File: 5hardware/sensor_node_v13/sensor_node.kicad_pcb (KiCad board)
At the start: 2 copper layers, 24 x 48 mm, 43 parts, among them J1 Conn_01x08_Socket, J2 Conn_01x08_Socket, Q1 AO3400A, Q2 AO3401A, Q4 AO3401A, SW1 SW_Push, SW2 SW_Push, SW3 SW_Push, SW4 SW_Reed, SW5 SW_Push, SW6 SW_Push, SW7 SW_Push, U1 ESP-12F, U12 APDS-9960, U13 SHT31-DIS, U17 BH1750FVI-TR, U2 2N7002DW, U3 INA219AxDCN, U7 XC6206PxxxMR, U8 TPL5110

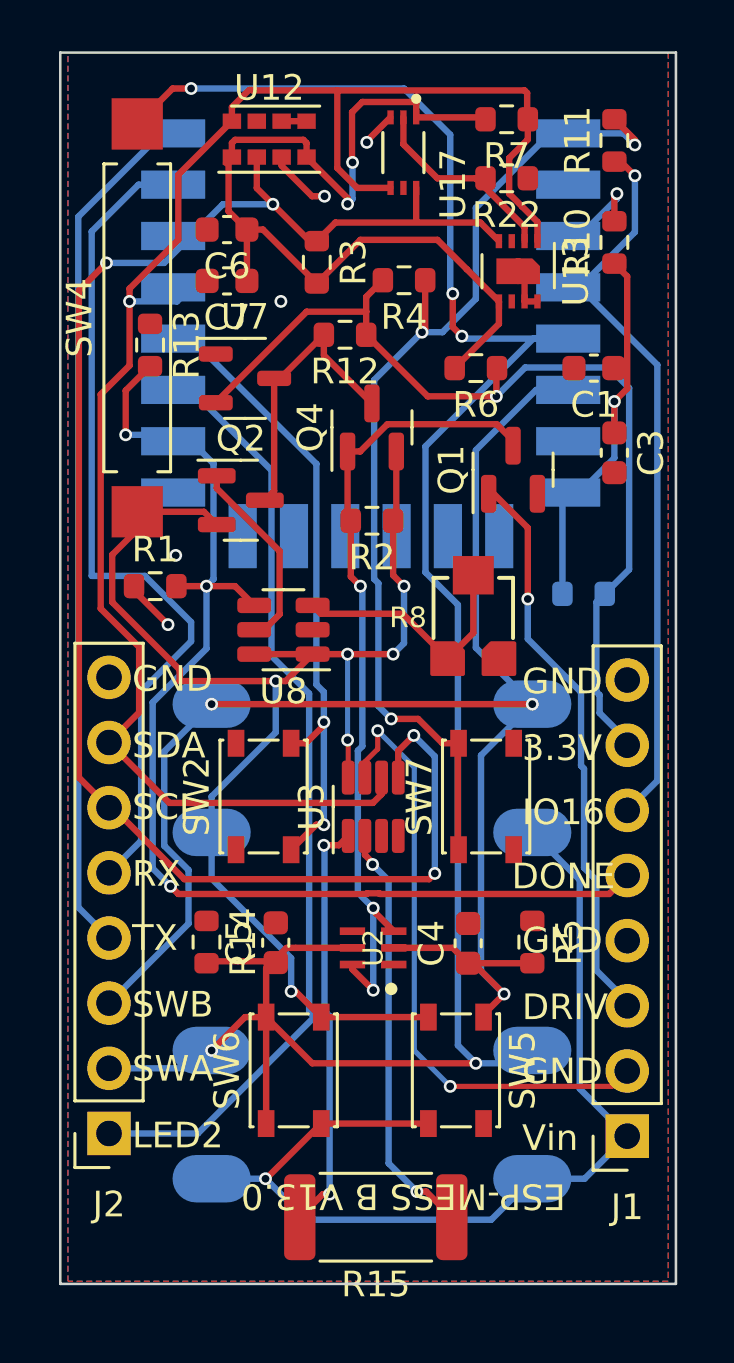
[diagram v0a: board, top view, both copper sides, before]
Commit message: updated PCB.
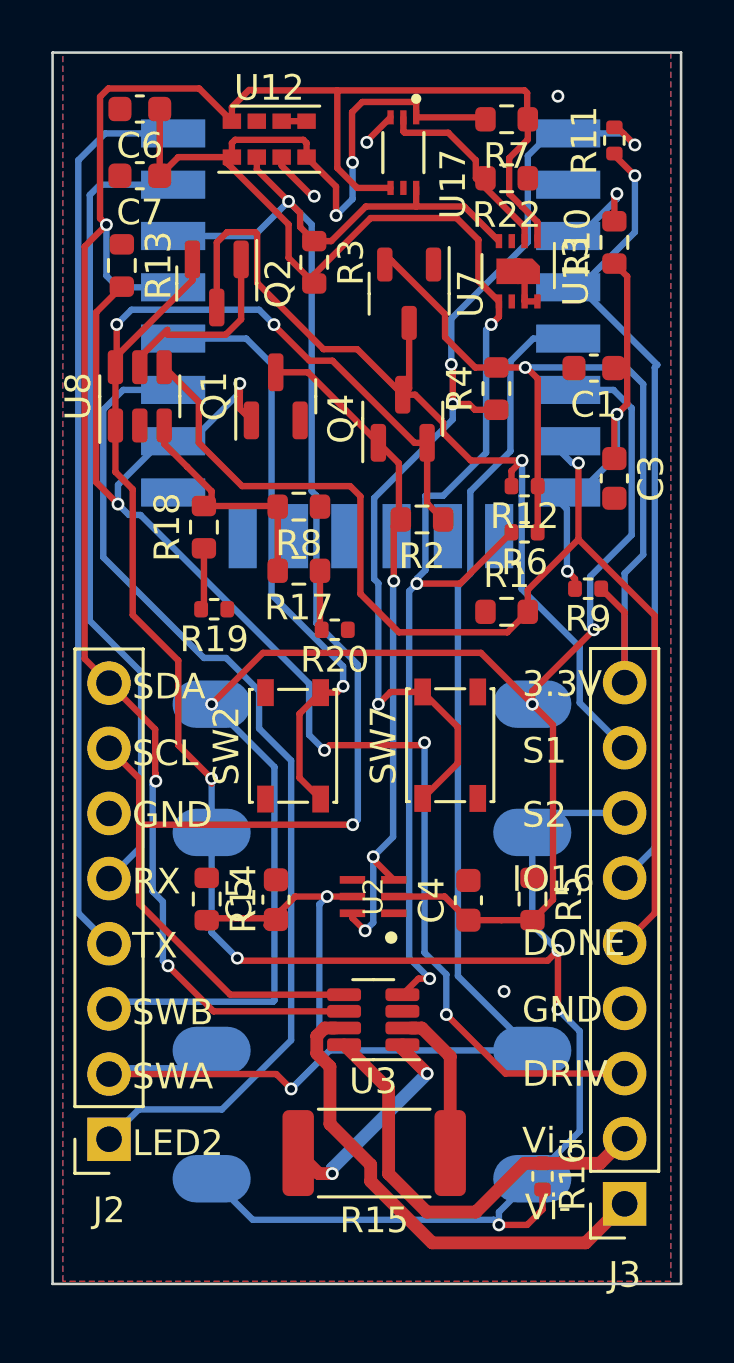
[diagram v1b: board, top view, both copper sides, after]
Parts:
- removed J1: Conn_01x08_Socket, Connector_PinSocket_2.54mm:PinSocket_1x08_P2.54mm_Vertical
- removed SW4: SW_Reed, Button_Switch_SMD:SW_SPST_REED_CT10-XXXX-G1
- removed SW5, SW6: SW_Push, Button_Switch_SMD:SW_SPST_PTS810
- added J3: Conn_01x09_Socket, Connector_PinSocket_2.54mm:PinSocket_1x09_P2.54mm_Vertical, F.Cu at (134.7, 98.8)
- added R16: 0K, Resistor_SMD:R_0402_1005Metric, F.Cu at (131.5, 97.7)
- added R17: R, Resistor_SMD:R_0603_1608Metric, F.Cu at (122.0, 74.1)
- added R18: R, Resistor_SMD:R_0603_1608Metric, F.Cu at (118.3, 72.4)
- added R19: 0K, Resistor_SMD:R_0402_1005Metric, F.Cu at (118.7, 75.6)
- added R20: 0K, Resistor_SMD:R_0402_1005Metric, F.Cu at (123.4, 76.4)
- R11, R12, R6: footprint Resistor_SMD:R_0603_1608Metric -> Resistor_SMD:R_0402_1005Metric
- R8: value EVM3ESX50B12 -> R; footprint EVM3ES:EMV3ESX50B12 -> Resistor_SMD:R_0603_1608Metric
- R9: footprint Resistor_SMD:R_0603_1608Metric -> Resistor_SMD:R_0402_1005Metric; moved to F.Cu
- moved R1 13.7 mm to (130.1, 75.7)
- moved U8 10.7 mm to (115.8, 67.3), turned to 90 degrees
- moved Q1 9.68 mm to (121.1, 67.3)
- moved R12 9.15 mm to (130.8, 70.8)
- moved Q2 8.50 mm to (118.8, 62.9), turned to -90 degrees
- moved U3 8.30 mm to (124.9, 91.6), turned to 180 degrees
- moved R8 8.06 mm to (122.0, 71.6), turned to 180 degrees
- moved U7 7.20 mm to (126.3, 63.3), turned to -90 degrees
- moved R6 6.68 mm to (130.8, 72.6)
- moved C6 5.80 mm to (115.8, 56.1)
- moved R4 5.55 mm to (129.7, 67.0), turned to 90 degrees
- moved C7 5.33 mm to (115.8, 58.7)
- moved R13 3.29 mm to (115.1, 62.2)
- moved R15 2.50 mm to (124.9, 96.8)
- moved SW7 2.44 mm to (127.9, 80.9)
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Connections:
- net Net-(Q2-D) renamed S1
- J2 pad 6: SCL -> GND
- J2 pad 7: SDA -> SCL
- J2 pad 8: GND -> SDA
- Q2 pad 2: Vi- -> S2
- Q4 pad 2: Vi- -> S2
- R2 pad 1: Vi- -> S2
- R8 pad 1: Net-(U8-DELAY/M_DRV) -> GND
- SW1 pad 1: Vi- -> S2
- SW3 pad 1: Vi- -> S2
- U8 pad 1: Vi- -> S2
- U8 pad 6: Vi- -> S2
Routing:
- net S2: track 0.00 -> 98.5 mm, vias 0 -> 7
- net Vi-: track 93.2 -> 16.2 mm, vias 7 -> 0
- net V-SENS: track 37.4 -> 74.6 mm, vias 2 -> 5
- net DRIVE: track 22.4 -> 54.7 mm, vias 1 -> 5
- net S1: track 11.0 -> 36.4 mm, vias 0 -> 1
- net SW-A: track 87.7 -> 67.0 mm, vias 5 -> 2
- net SDA: track 66.7 -> 78.9 mm, vias 1 -> 3
- net Net-(U3-IN-): track 16.5 -> 5.75 mm, vias 2 -> 0
- net Net-(U3-IN+): track 16.3 -> 8.61 mm
- net Vi+: track 24.2 -> 18.9 mm, vias 2 -> 0
- net Net-(Q1-D): track 31.5 -> 27.2 mm
- net LED2: track 36.3 -> 40.6 mm
- net IO16: track 29.4 -> 32.4 mm
- net SCL: track 64.5 -> 67.4 mm, vias 4 -> 2
- net SW-B: track 62.2 -> 64.7 mm
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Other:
- board size 24 x 48 mm -> 24.5 x 48 mm
- board text added: "ESP-MESS B V13.2"
- board text added: "S1"
- board text added: "S2"
- board text added: "Vi+"
- board text added: "Vi-"
- board text removed: "ESP-MESS B V13.0"
- board text removed: "Vin"
